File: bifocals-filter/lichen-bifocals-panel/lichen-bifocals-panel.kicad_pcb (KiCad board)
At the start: 2 copper layers, 40.3 x 128.5 mm, 20 parts

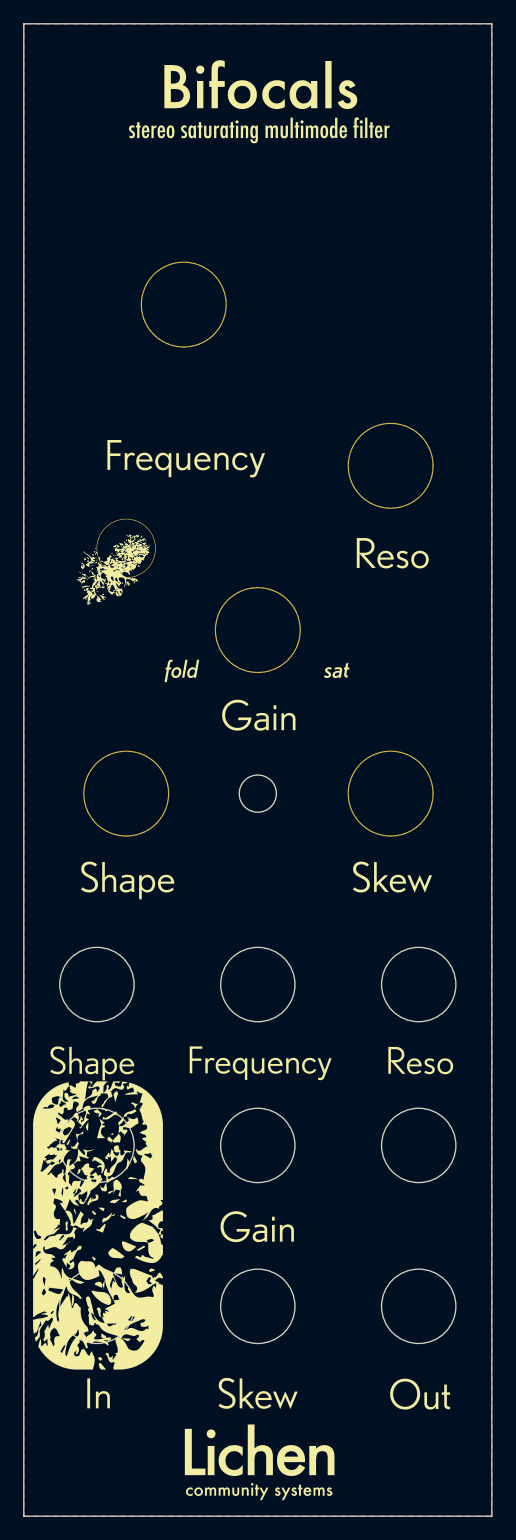
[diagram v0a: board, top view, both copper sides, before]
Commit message: v1.1 of Freddie and Bifocals hardware.
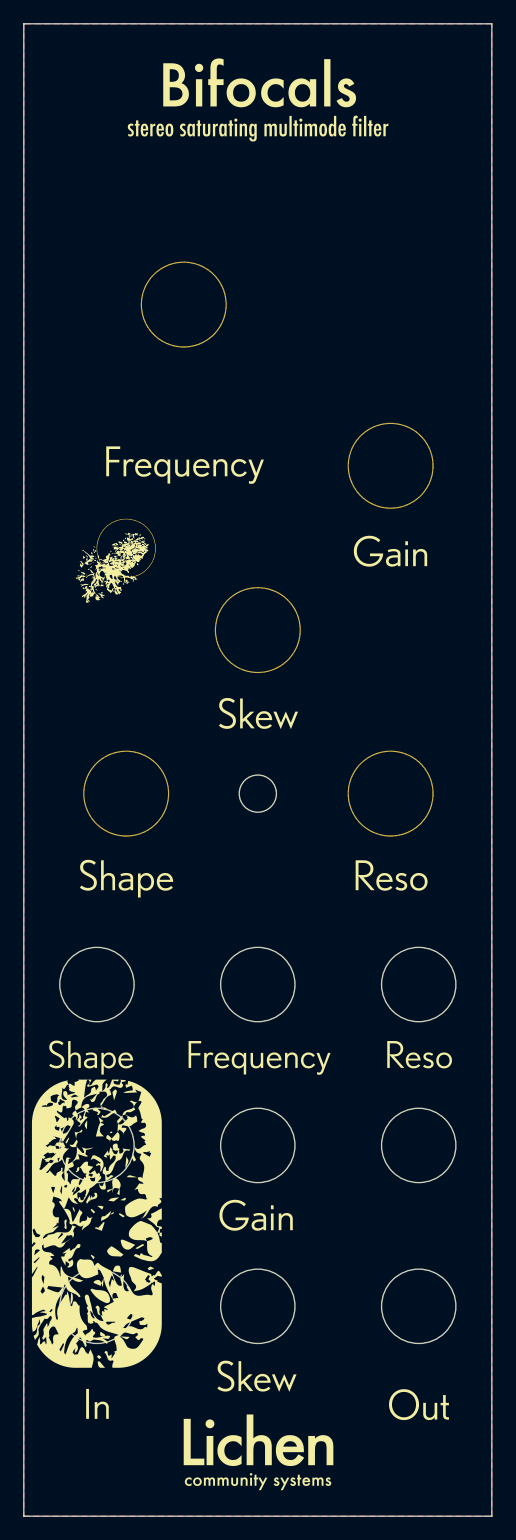
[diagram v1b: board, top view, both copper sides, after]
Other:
- board text added: "August 2024"
- board text added: "Lichen Bifocals v1.1"
- board text removed: "February 2024"
- board text removed: "Lichen Bifocals v1.0"
